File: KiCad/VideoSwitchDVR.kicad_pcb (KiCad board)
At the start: 2 copper layers, 18 x 25 mm, 25 parts, among them J1 EV100, J2 Buttons, J3 DVR_VIDEO, J4 PWR, J5 PWR_DVR, J6 PROG, Q1 AO3415 (P), U1 ATTINY15-1SC, U2 MAX4624/5

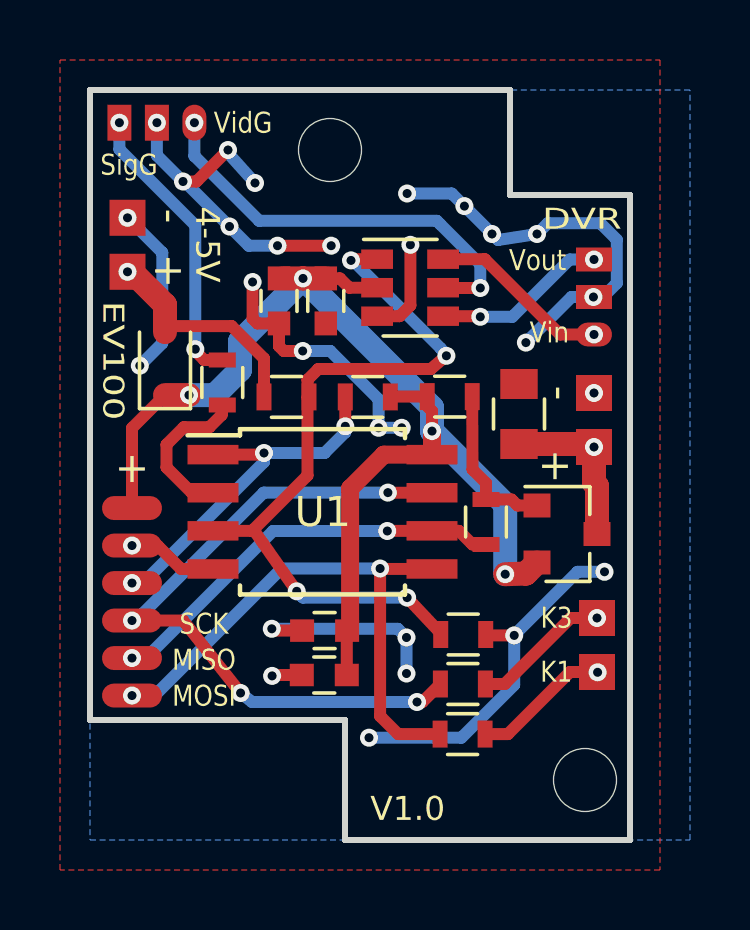
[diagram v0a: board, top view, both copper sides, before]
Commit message: PCB 2.0. Case SCAD.
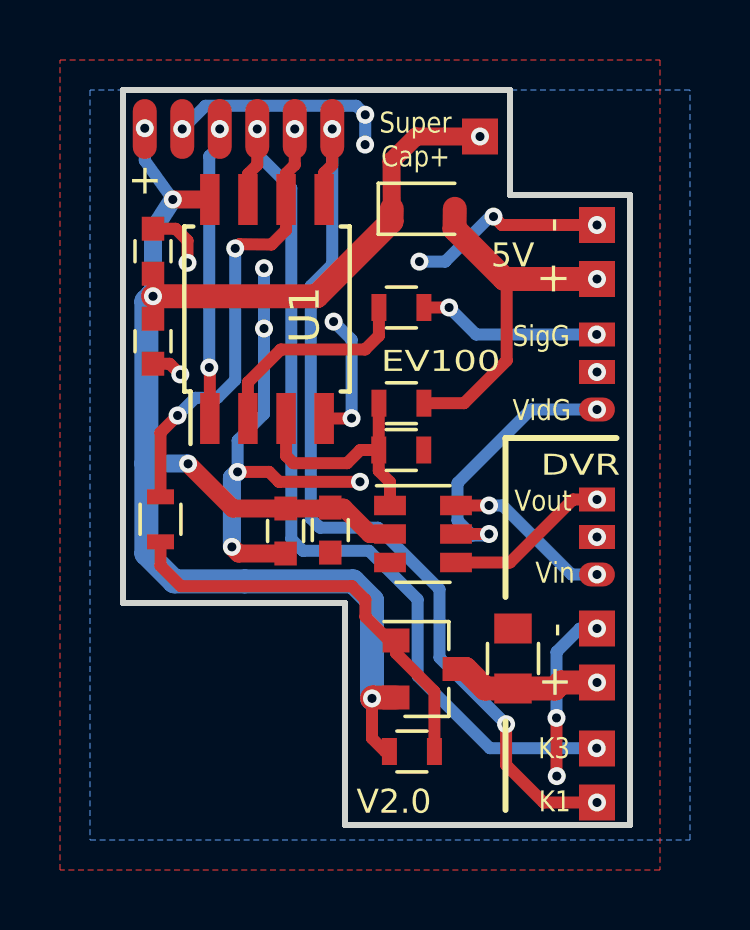
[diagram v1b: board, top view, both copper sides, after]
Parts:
- removed R1, R3: 100, Resistors_SMD:R_0603
- removed R5: 10K, Resistors_SMD:R_0603
- removed REF** (x2): MountingHole_2.2mm_M2, Mounting_Holes:MountingHole_2.2mm_M2
- added J7: SuperCap, KiCadCustomLibs:ESC_PWR_PAD, F.Cu at (113.0, 81.5)
- U1: value ATTINY15-1SC -> ATTINY25
- moved J1 16.9 mm to (116.9, 89.4), turned to 90 degrees
- moved J6 16.2 mm to (105.0, 81.3), turned to 180 degrees
- moved J4 15.7 mm to (116.9, 85.4)
- moved C2 15.2 mm to (102.1, 85.4), turned to 90 degrees
- moved R2 11.9 mm to (110.7, 102.0)
- moved C1 11.2 mm to (102.1, 88.4), turned to 270 degrees
- moved R6 10.9 mm to (102.3, 94.3), turned to 270 degrees
- moved D1 10.0 mm to (111.1, 84.0), turned to 0 degrees
- moved U2 8.22 mm to (111.1, 94.8)
- moved C5 8.15 mm to (114.1, 99.0)
- moved J3 8.00 mm to (116.9, 94.9)
- moved J5 7.85 mm to (116.9, 98.8)
- moved C4 7.67 mm to (106.5, 94.7)
- moved C3 7.64 mm to (108.0, 94.7)
- moved U1 7.01 mm to (105.9, 87.3), turned to 90 degrees
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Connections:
- J2 pad 1: /K3 -> /SCK
- J2 pad 2: /K1 -> /MOSI
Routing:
- net GND: track 65.9 -> 43.4 mm, vias 29 -> 20
- net /VID_SWITCH: track 25.7 -> 8.19 mm, vias 4 -> 0
- net VCC: track 40.8 -> 55.4 mm, vias 4 -> 6
- net /MOSI: track 19.0 -> 31.3 mm, vias 2 -> 3
- net Net-(Q1-Pad1): track 5.40 -> 14.3 mm
- net /SCK: track 23.6 -> 31.2 mm, vias 4 -> 2
- net /K3: track 5.06 -> 0.00 mm, vias 1 -> 0
- net Net-(J1-Pad1): track 14.2 -> 9.29 mm
- net /K1: track 4.59 -> 0.00 mm, vias 1 -> 0
- net +5V: track 8.02 -> 12.2 mm
- net /VID_SENSE: track 10.0 -> 6.14 mm
- net /RST: track 12.4 -> 9.80 mm, vias 3 -> 2
- net Net-(R4-Pad2): track 5.24 -> 7.15 mm
- net /MISO: track 13.7 -> 15.2 mm, vias 2 -> 3
- net Net-(J3-Pad1): track 6.08 -> 5.65 mm, vias 1 -> 2
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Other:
- board size 18 x 25 mm -> 16.9 x 24.5 mm
- board text added: "5V"
- board text added: "RST"
- board text added: "Super Cap+"
- board text added: "V2.0"
- board text removed: "4-5V"
- board text removed: "V1.0"
